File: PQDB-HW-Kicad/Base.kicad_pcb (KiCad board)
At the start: 2 copper layers, 146.1 x 141 mm, 71 parts, among them Q101 BC847, Q102 BC847, Q201 BC847, Q301 BC847, Q302 BC847, Q303 BC847, Q304 BC847, SW101 BTN-01, SW102 BTN-01, SW103 BTN-01, SW104 BTN-01, SW105 BTN-01, SW106 BTN-01, SW107 BTN-01, SW108 BTN-01, SW109 BTN-01, SW110 BTN-01, U201 LM35, U301 KW4-361, U401 DISPLAY_JHD162A, U601 74HC595, U701 DS1307Z, X701 32.768 KHz

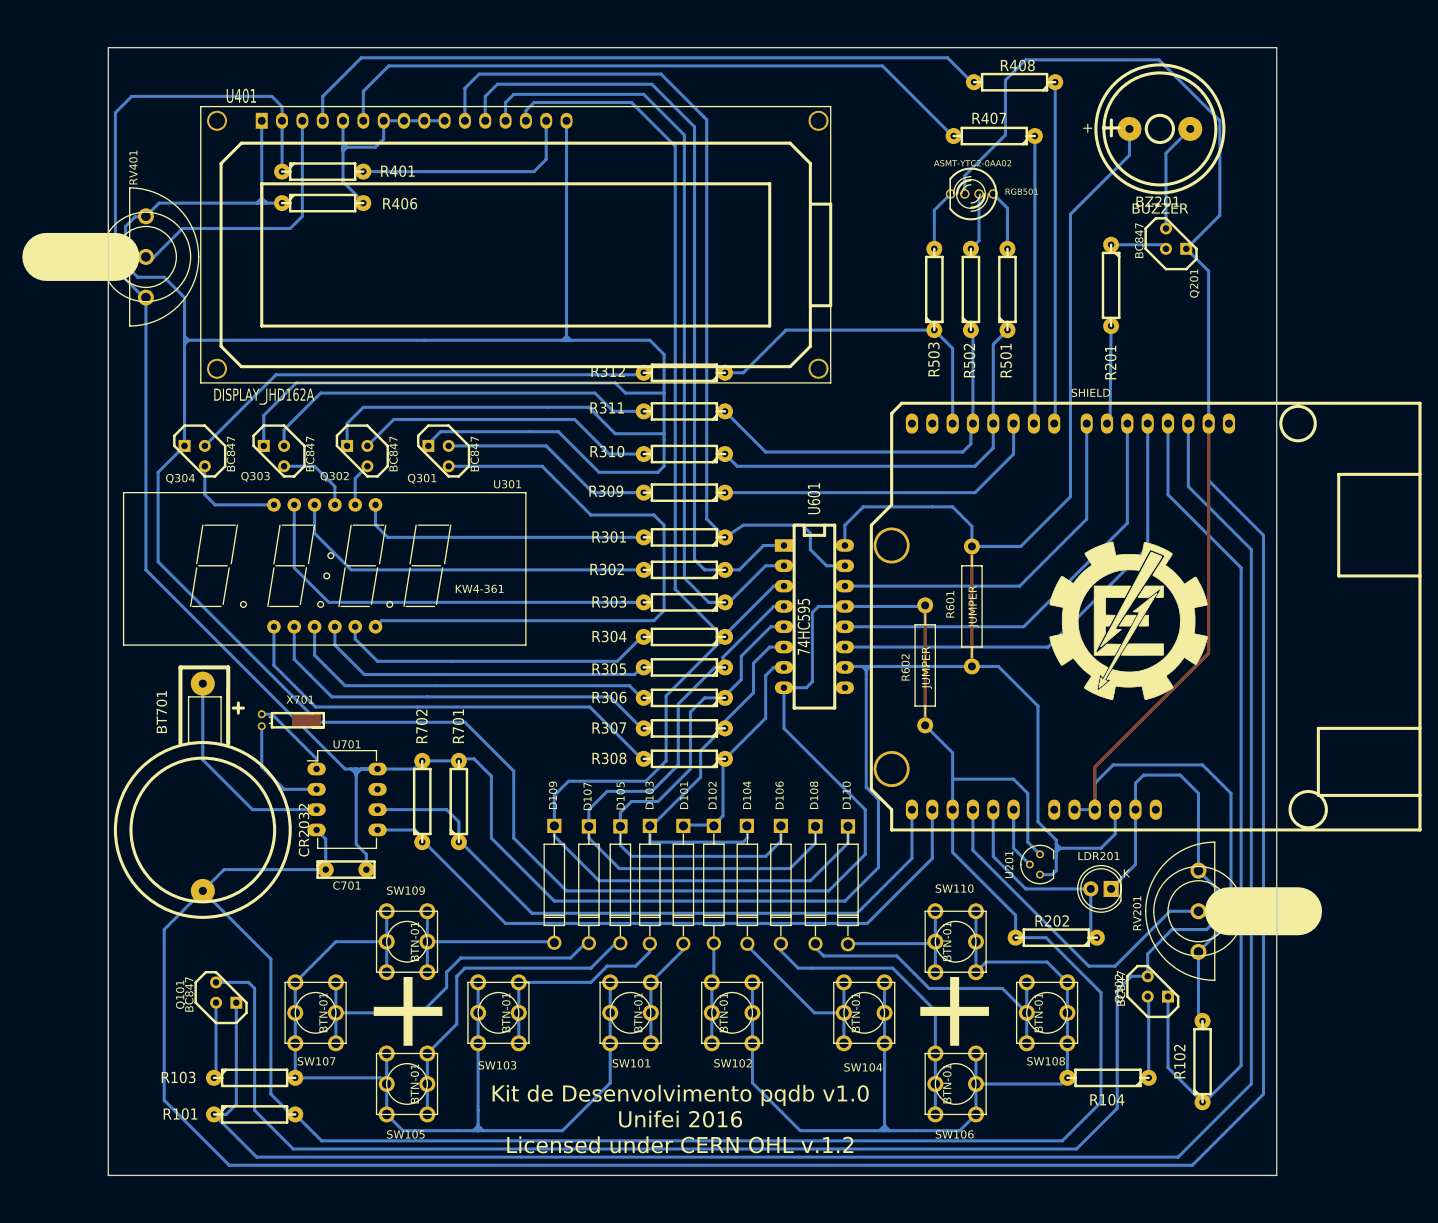
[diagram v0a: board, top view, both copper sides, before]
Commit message: Add files via upload
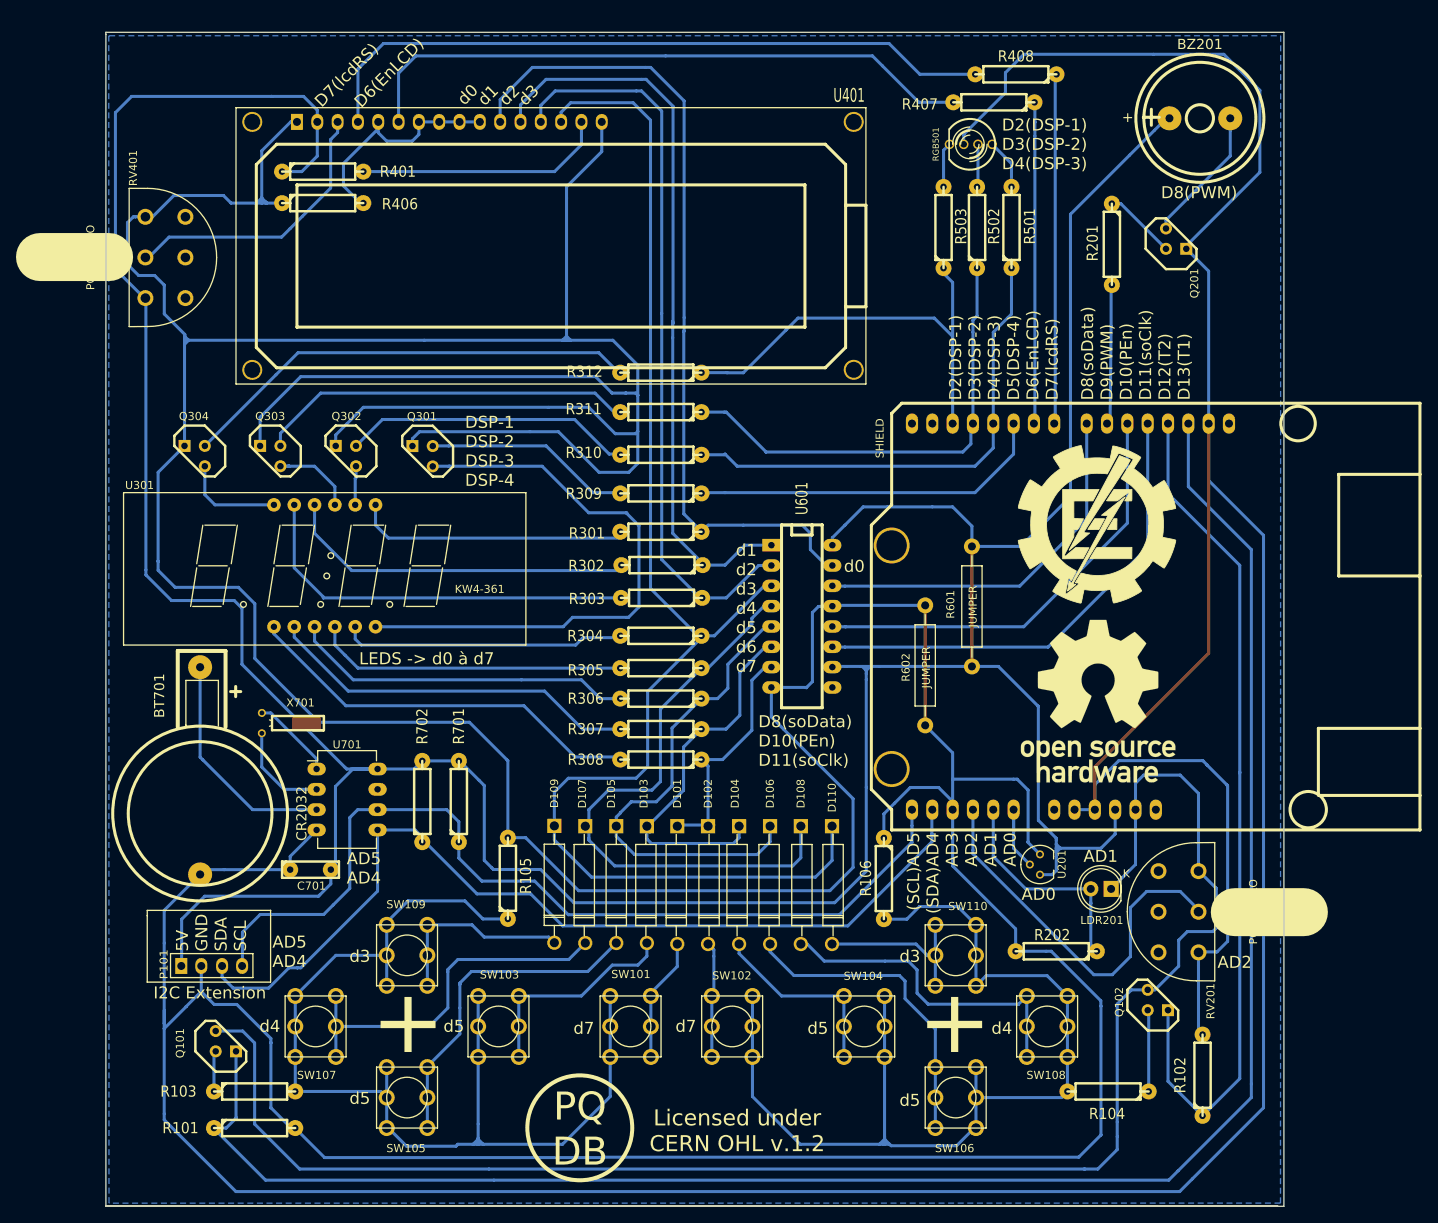
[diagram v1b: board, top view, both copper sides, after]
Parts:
- added G***: LOGO, bibliotecas:OSHW_GRANDE, F.Cu at (181.5, 104.6)
- added P101: EXT_I2C, bibliotecas:EXT_I2C, F.Cu at (65.8, 139.1)
- added R105: 1k, bibliotecas:HW_Resistor, F.Cu at (107.7, 126.7)
- added R106: 1k, bibliotecas:HW_Resistor, F.Cu at (154.7, 126.7)
- G***: moved to F.Cu
- RV201, RV401: value POT -> POT_DUPLO; footprint HW_Potenciometro_2 -> bibliotecas:HW_Potenciometro_2_Duplo
- X701: footprint Crystals:Crystal_Round_Horizontal_2mm -> bibliotecas:Crystal_Round_Horizontal_2mm
- moved G*** 12.7 mm to (181.2, 82.4)
- moved R503 7.83 mm to (162.2, 45.3)
- moved R502 7.78 mm to (166.4, 45.3)
- moved R501 7.77 mm to (170.7, 45.3)
- moved RGB501 6.21 mm to (165.7, 34.9)
- moved Q101 6.08 mm to (72.5, 147.1)
- moved BZ201 5.17 mm to (194.2, 31.7)
- moved R201 5.14 mm to (183.2, 47.4)
- moved C701 4.45 mm to (83.1, 125.6)
- moved U401 4.41 mm to (75.8, 32.1)
- moved R407 4.22 mm to (168.5, 29.7)
- moved R301 3.02 mm to (126.9, 83.4)
- moved R312 2.95 mm to (126.8, 63.5)
- moved R305 2.94 mm to (126.9, 100.4)
- moved R306 2.94 mm to (126.9, 104.2)
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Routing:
- net +5V: track 416.2 -> 461.6 mm
- net /SDA: track 84.4 -> 118.6 mm
- net GND: track 1193.9 -> 1226.8 mm
- net /SCL: track 82.4 -> 115.2 mm
- net Net-(R103-Pad2): track 117.1 -> 134.9 mm
- net /DSP-1: track 40.7 -> 55.4 mm
- net Net-(R104-Pad2): track 116.7 -> 130.0 mm
- net /DSP-2: track 47.8 -> 59.0 mm
- net /DSP-3: track 50.6 -> 61.5 mm
- net /D3: track 179.6 -> 172.1 mm
- net /AN2: track 42.1 -> 49.1 mm
- net /D1: track 99.1 -> 92.8 mm
- net /D2: track 98.8 -> 92.5 mm
- net /D0: track 109.3 -> 103.4 mm
- net /PWM: track 12.4 -> 17.6 mm
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- added copper zone on B.Cu, net (none)
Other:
- board size 146.1 x 141 mm -> 147.2 x 146.8 mm
- net class Default: clearance 0.762 -> 0.5
- rule trace_clearance: 0.762 -> 0.5
- board text added: "(SCL)AD5 (SDA)AD4 AD3 AD2 AD1 AD0"
- board text added: "5V GND SDA SCL"
- board text added: "AD0"
- board text added: "AD1"
- board text added: "AD2"
- board text added: "AD5 AD4"
- board text added: "D2(DSP-1) D3(DSP-2) D4(DSP-3)"
- board text added: "D2(DSP-1) D3(DSP-2) D4(DSP-3) D5(DSP-4) D6(EnLCD) D7(lcdRS)"
- board text added: "D6(EnLCD)"
- board text added: "D7(lcdRS)"
- board text added: "D8(PWM)"
- board text added: "D8(soData) D10(PEn) D11(soClk)"
- board text added: "D8(soData) D9(PWM) D10(PEn) D11(soClk) D12(T2) D13(T1)"
- board text added: "DSP-1 DSP-2 DSP-3 DSP-4"
- board text added: "I2C Extension"
- board text added: "LEDS -> d0 à d7"
- board text added: "Licensed under CERN OHL v.1.2"
- board text added: "PQ DB"
- board text added: "d0"
- board text added: "d1"
- board text added: "d1 d2 d3 d4 d5 d6 d7"
- board text added: "d2"
- board text added: "d3"
- board text added: "d4"
- board text added: "d5"
- board text added: "d7"
- board text removed: "Kit de Desenvolvimento pqdb v1.0 Unifei 2016 Licensed under CERN OHL v.1.2"
